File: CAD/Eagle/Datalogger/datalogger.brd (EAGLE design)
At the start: 27.9 x 83.8 mm, 8 parts

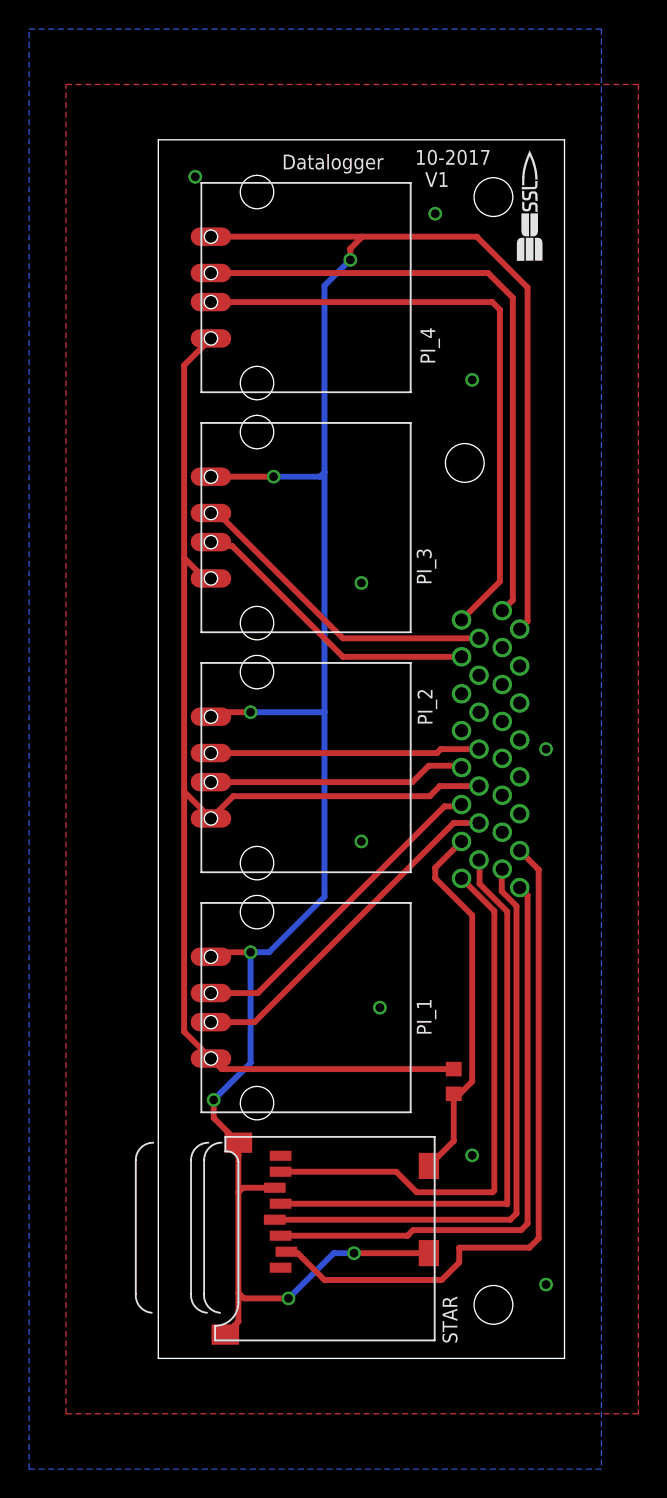
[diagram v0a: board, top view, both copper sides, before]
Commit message: datalogger eagle and NX
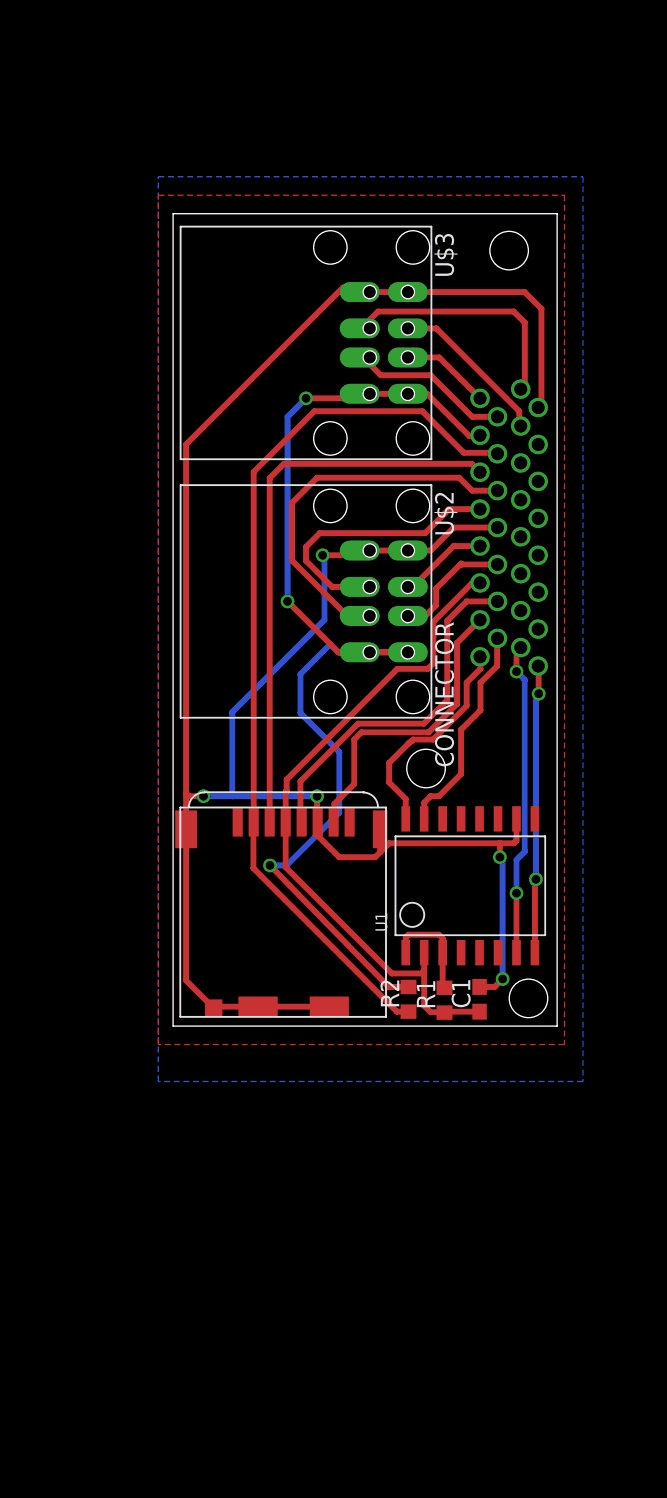
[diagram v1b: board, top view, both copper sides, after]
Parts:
- removed PI_1, PI_2, PI_3, PI_4: USB_A, NR_connectors:USB_A
- removed R5: (no value), resistor:R0603
- removed STAR: MICROSD, adafruit:MICROSD
- added C1: 100nF, resistor:C0603
- added R1: 4.7k, resistor:R0603
- added R2: (no value), resistor:R0603
- added U$2, U$3: USB_A, NR_connectors:USB_A
- added U1: MT25QL01GBBB8ESF-0AAT, NR_IC:SOP2-16
- U$1: value SSL.3IN_SILK -> MICRO_SD; device images:SSL_SILK_.3IN -> NR_connectors:MICRO_SD_HINGED
- moved U$1 55.3 mm to (-8.51, -14.6), turned to 180 degrees
- moved CONNECTOR 15.3 mm to (10.2, 19.1)
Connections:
- removed net CS_STAR: CONNECTOR.3, STAR.2
- removed net D: CONNECTOR.25
- removed net FOUR: CONNECTOR.11
- removed net N$7: CONNECTOR.12
- removed net N$8: CONNECTOR.13
- removed net ONE: CONNECTOR.27
- removed net R: CONNECTOR.26
- removed net THREE: CONNECTOR.10
- removed net TWO: CONNECTOR.28
- new net MISO_FLASH: CONNECTOR.1, U1.8
- new net MOSI_FLASH: CONNECTOR.18, U1.15
- new net N$1: R1.2, U1.1, U1.3
- new net PB23: CONNECTOR.2, U1.7
- new net SCK_FLASH: CONNECTOR.17, U1.16
- net +3V3: now also C1.1, CONNECTOR.21, R1.1, U$1.VDD, U1.2; no longer CONNECTOR.2, STAR.4
- net +5V: now also CONNECTOR.29, R2.2, U$2.VCC1, U$2.VCC2, U$3.VCC1, U$3.VCC2; no longer CONNECTOR.22, PI_1.VCC, PI_2.VCC, PI_3.VCC, PI_4.VCC, R5.2
- net DATA+1: now also CONNECTOR.23, U$2.DATA+1; no longer CONNECTOR.21, PI_1.DATA+
- net DATA+2: now also CONNECTOR.25, U$2.DATA+2; no longer CONNECTOR.24, PI_2.DATA+
- net DATA+3: now also CONNECTOR.14, U$3.DATA+1; no longer CONNECTOR.30, PI_3.DATA+
- net DATA+4: now also U$3.DATA+2; no longer PI_4.DATA+
- net DATA-1: now also CONNECTOR.22, U$2.DATA-1; no longer CONNECTOR.20, PI_1.DATA-
- net DATA-2: now also CONNECTOR.26, U$2.DATA-2; no longer CONNECTOR.23, PI_2.DATA-
- net DATA-3: now also CONNECTOR.31, U$3.DATA-1; no longer CONNECTOR.29, PI_3.DATA-
- net DATA-4: now also CONNECTOR.30, U$3.DATA-2; no longer CONNECTOR.31, PI_4.DATA-
- net GND: now also C1.2, CONNECTOR.24, U$1.CD1, U$1.GND1, U$1.GND2, U$1.GND3, U$1.GND4, U$1.VSS, U$2.GND1, U$2.GND2, U$3.GND1, U$3.GND2, U1.10; no longer PI_1.GND, PI_2.GND, PI_3.GND, PI_4.GND, STAR.6, STAR.CD2, STAR.MT1, STAR.MT2
- net MISO_STAR: now also CONNECTOR.27, U$1.CMD; no longer CONNECTOR.17, STAR.7
- net MOSI_STAR: now also CONNECTOR.19, U$1.DAT0; no longer CONNECTOR.1, STAR.3
- net SCK_STAR: now also CONNECTOR.20, U$1.CLK; no longer CONNECTOR.18, STAR.5
- net SD_STAR: now also CONNECTOR.28, R2.1, U$1.CD; no longer CONNECTOR.19, R5.1, STAR.CD1
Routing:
- net CS_STAR: track 47.1 -> 0.00 mm
- net SD_STAR: track 25.6 -> 61.7 mm
- net DATA-4: track 42.5 -> 10.7 mm
- net DATA+4: track 43.3 -> 16.5 mm
- net PB23: track 0.00 -> 21.6 mm, vias 0 -> 2
- net MOSI_STAR: track 40.7 -> 20.8 mm
- net MISO_FLASH: track 0.00 -> 19.8 mm, vias 0 -> 2
- net +5V: track 92.8 -> 73.9 mm, vias 0 -> 3
- net DATA+1: track 22.6 -> 6.13 mm
- net DATA-1: track 24.1 -> 8.35 mm
- net SCK_STAR: track 40.1 -> 24.8 mm
- net SCK_FLASH: track 0.00 -> 15.1 mm
- net MOSI_FLASH: track 0.00 -> 14.8 mm
- net DATA-3: track 20.5 -> 6.13 mm
- net DATA+3: track 22.0 -> 11.1 mm
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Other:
- board size 27.9 x 83.8 mm -> 26.4 x 55.9 mm
- board text removed: "10-2017"
- board text removed: "Datalogger"
- board text removed: "V1"
